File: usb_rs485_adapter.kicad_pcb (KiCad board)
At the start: 2 copper layers, 35 x 35 mm, 28 parts, among them J1 USB_C_Receptacle_USB2.0_16P, J2 Conn_01x06_Pin, U1 MAX485E, U2 CH340E, U3 MAX485E

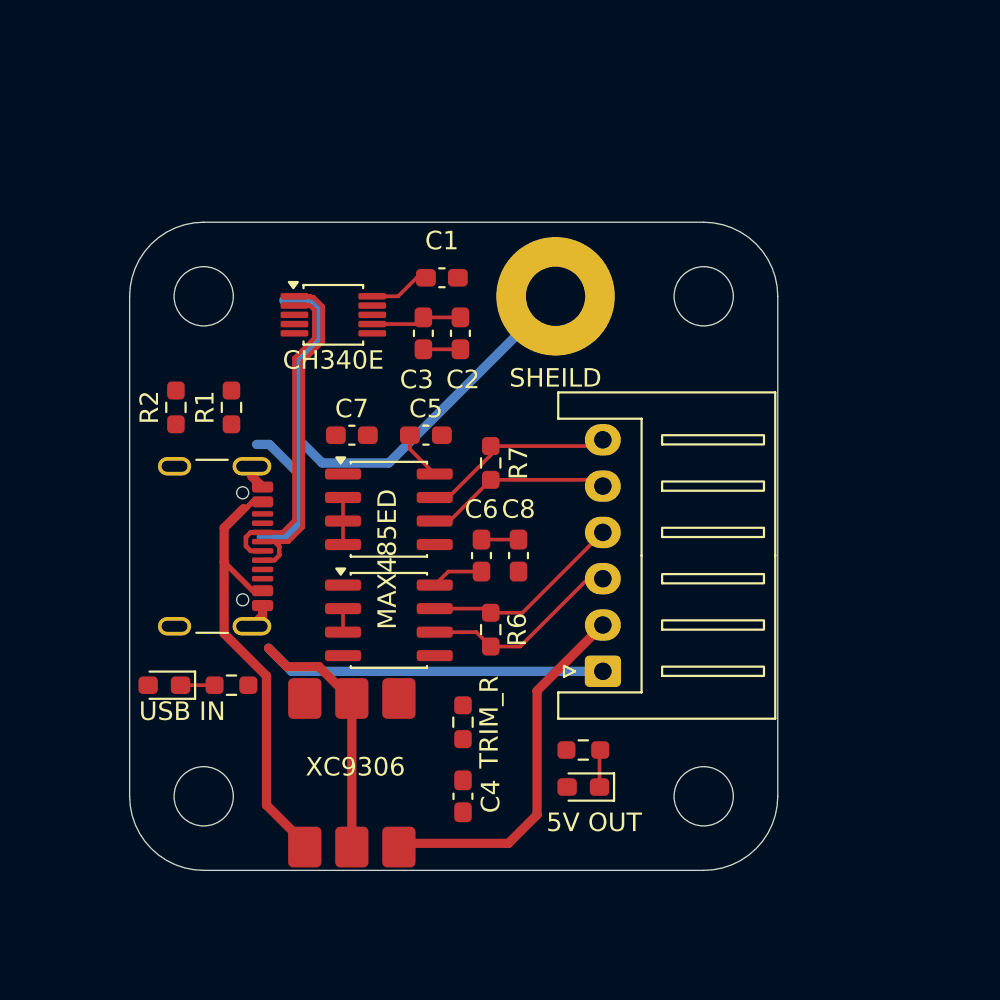
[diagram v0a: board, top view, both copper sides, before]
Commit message: パーツが基盤ギリギリ過ぎた
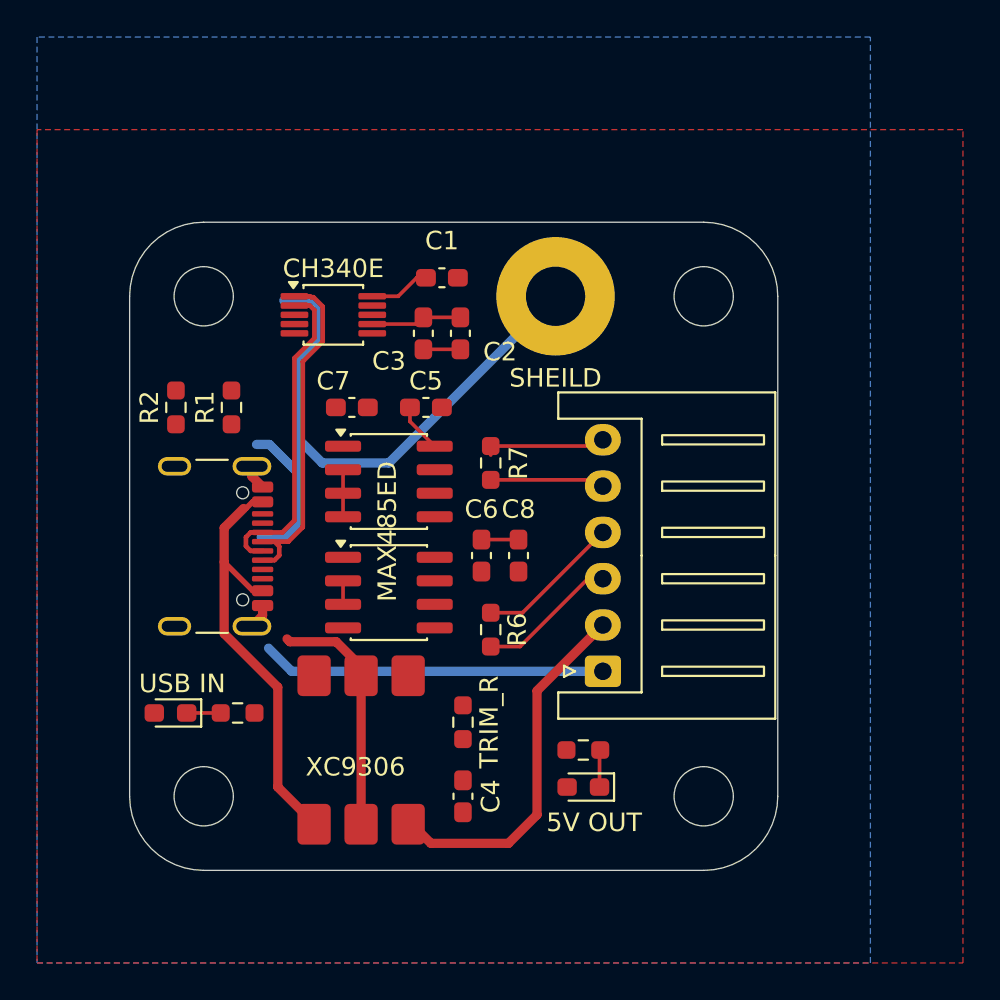
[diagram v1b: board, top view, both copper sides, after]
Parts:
- moved D1 1.54 mm to (102.2, 126.5)
- moved R3 1.54 mm to (105.8, 126.5)
- moved C5 1.50 mm to (116.0, 110.0)
- moved C7 1.50 mm to (112.0, 110.0)
- moved U1 1.50 mm to (114.0, 114.0)
- moved U3 1.50 mm to (114.0, 120.0)
- moved U4 1.33 mm to (112.5, 129.8)
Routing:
- net VCC: track 35.9 -> 32.1 mm
- net /TX+: track 10.9 -> 7.57 mm
- net /RX-: track 10.7 -> 7.42 mm
- net /RX+: track 10.1 -> 7.00 mm
- net /TX-: track 11.0 -> 8.17 mm
- added copper zone on B.Cu, net GND
- added copper zone on F.Cu, net GND
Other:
- board text added: "2026/09/07 Oinaru Board v1.0"
- board text added: "Takuto Ishihara ishiharanamazu@gmail.com"
- board text removed: "2026/09/07 Oinaru Board v1.0 Takuto Ishihara ishiharanamazu@gmail.com"

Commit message: v1.0完成
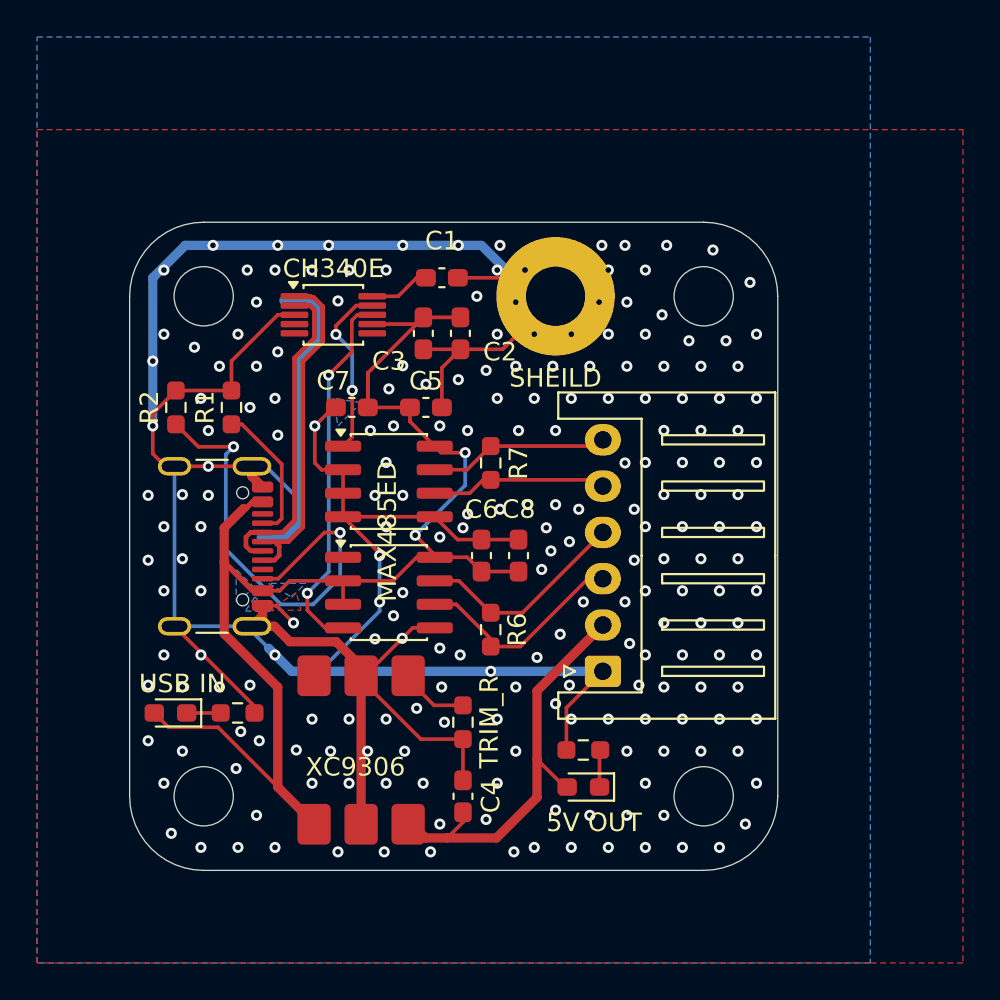
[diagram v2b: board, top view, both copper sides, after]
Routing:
- net GND: track 78.2 -> 194.3 mm, vias 0 -> 218
- net VCC: track 32.1 -> 74.6 mm, vias 0 -> 2
- net Net-(J1-CC2): track 0.00 -> 25.0 mm, vias 0 -> 2
- net /TXD: track 0.00 -> 20.2 mm, vias 0 -> 2
- net /RXD: track 0.00 -> 9.48 mm, vias 0 -> 2
- net Net-(J1-CC1): track 0.00 -> 7.68 mm
- net /TX+: track 7.57 -> 11.8 mm
- net +5V: track 19.8 -> 23.5 mm
- net Net-(U4-TRIM): track 0.00 -> 3.54 mm
- net /TX-: track 8.17 -> 11.6 mm
- net /RX+: track 7.00 -> 9.52 mm
- net /RX-: track 7.42 -> 9.75 mm

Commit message: シルク微修正
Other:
- board text added: "2026/09/07 Takuto Ishihara ishiharanamazu@gmail.com"
- board text added: "OinaruBoard v1.0"
- board text removed: "2026/09/07 Oinaru Board v1.0"
- board text removed: "Takuto Ishihara ishiharanamazu@gmail.com"
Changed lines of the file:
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@@
 		)
 	)
-	(gr_text "Takuto Ishihara\nishiharanamazu@gmail.com"
+	(gr_text "2026/09/07\nTakuto Ishihara\nishiharanamazu@gmail.com"
 		(at 127.5 134.5 0)
 		(layer "B.SilkS")
@@
 		)
 	)
-	(gr_text "2026/09/07\nOinaru Board v1.0"
-		(at 124.5 117.5 90)
+	(gr_text "OinaruBoard v1.0"
+		(at 123 117.5 90)
 		(layer "B.SilkS")
 		(effects
